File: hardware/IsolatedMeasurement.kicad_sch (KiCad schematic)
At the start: 27 parts, among them IC2 MCP3561T-E_NC, IC3 ADUM7441, IC6 AP7365-33YRG-13, IC9 REF193GSZ-REEL, P1 AM1LS-0505S-NZ

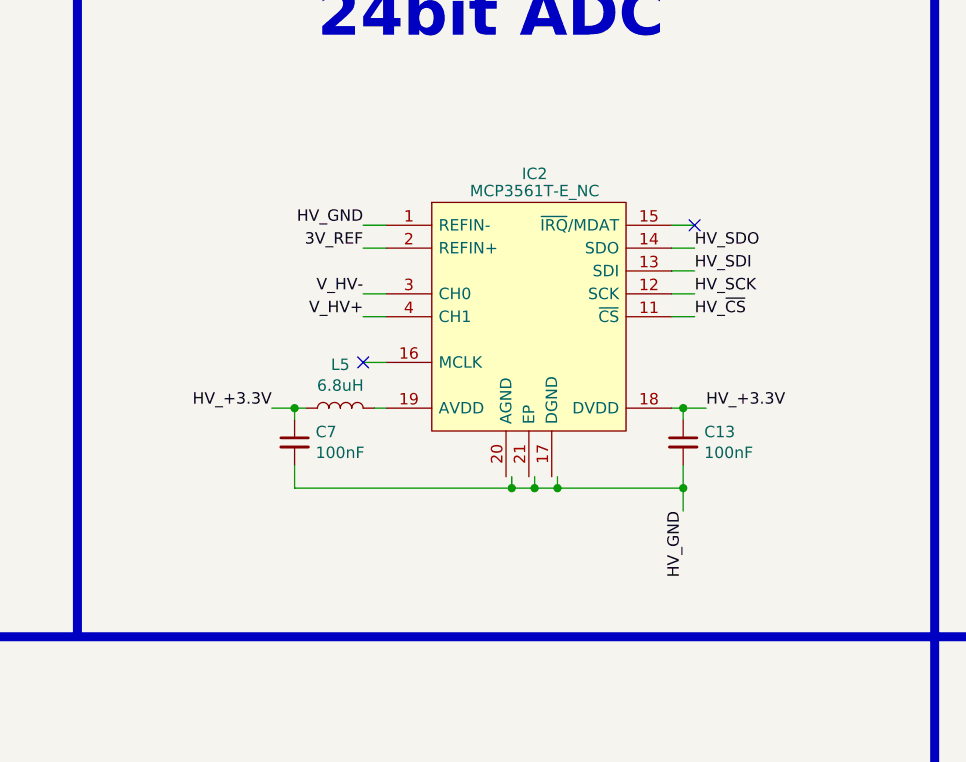
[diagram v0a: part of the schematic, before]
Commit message: done
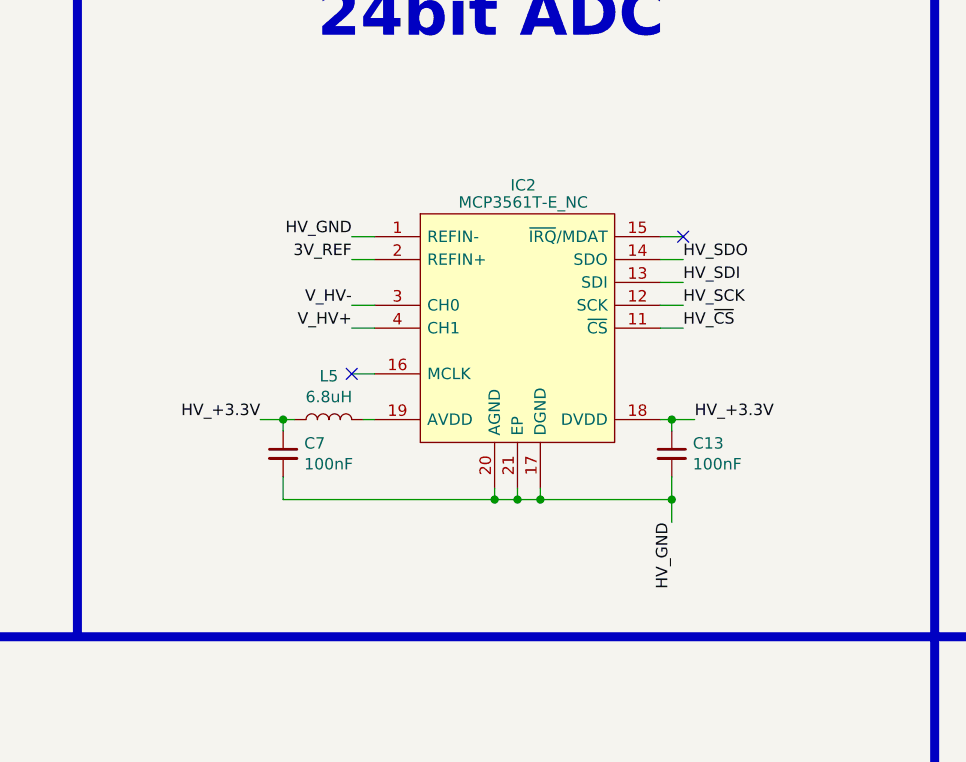
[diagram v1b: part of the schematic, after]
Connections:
- net HV_IN-: now also IC2.17 (DGND), IC2.20 (AGND), IC2.21 (EP)
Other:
- moved on the sheet: C13, C7, IC2, L5
